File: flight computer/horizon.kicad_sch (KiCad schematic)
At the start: 36 parts, among them J2 Conn_02x03_Counter_Clockwise, J7 Conn_02x03_Counter_Clockwise, J8 Conn_02x03_Counter_Clockwise, U1 MMCU, U3 NMCU, U4 TMCU, Y1 Crystal

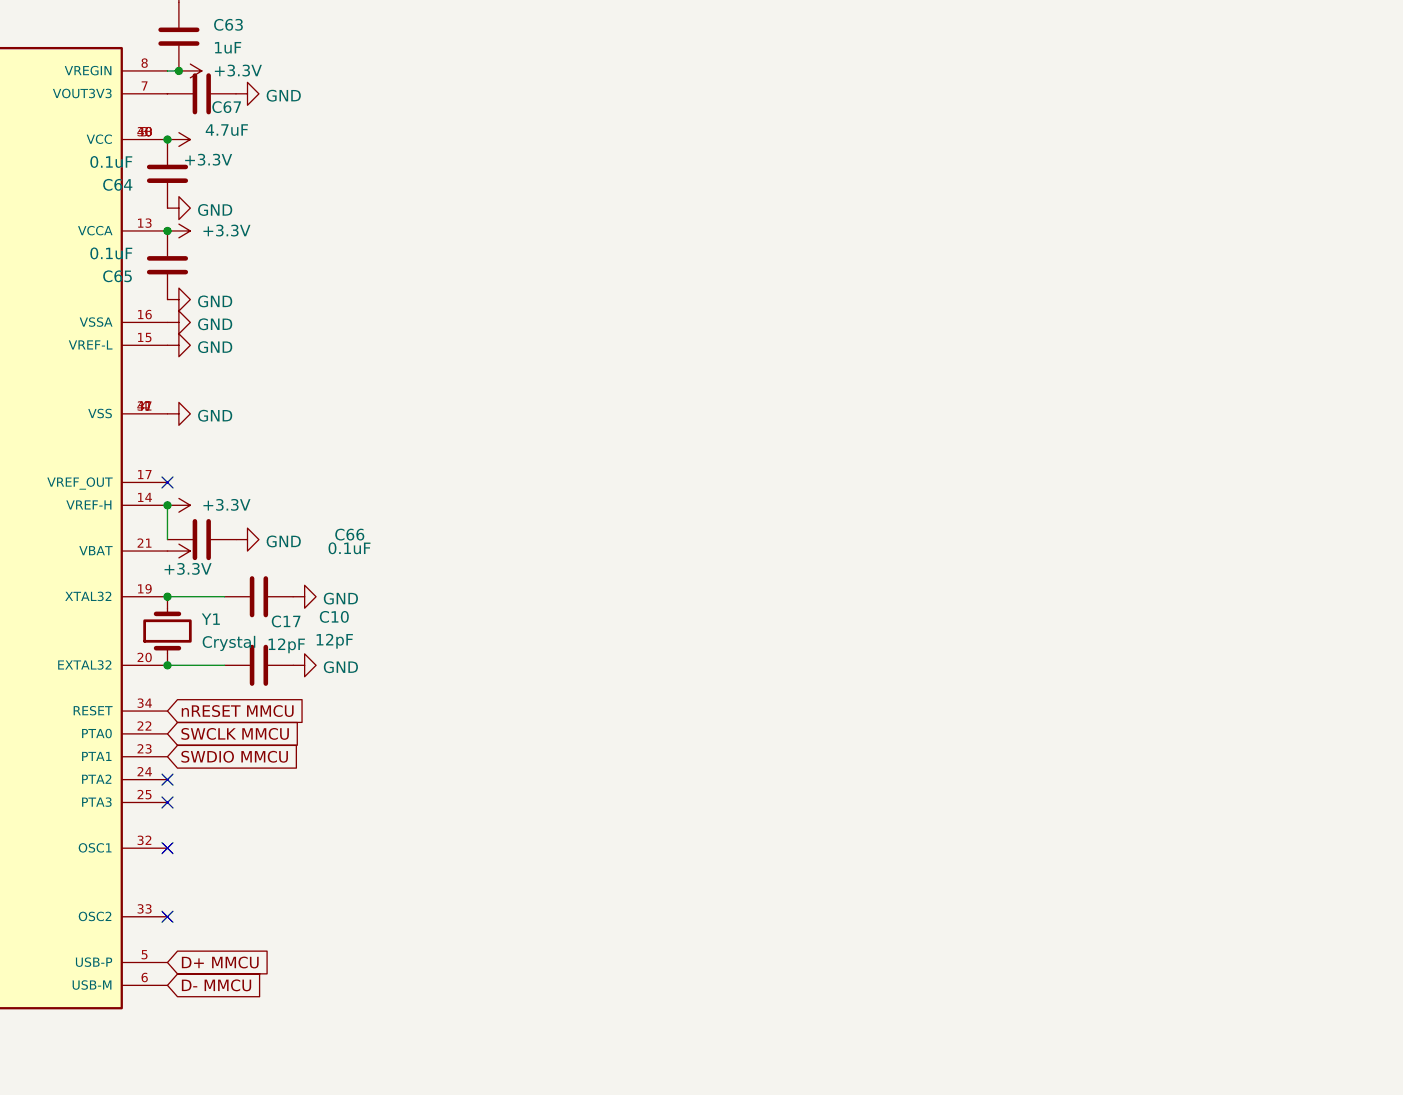
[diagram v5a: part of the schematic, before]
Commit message: Started wiring the teensy bootloader
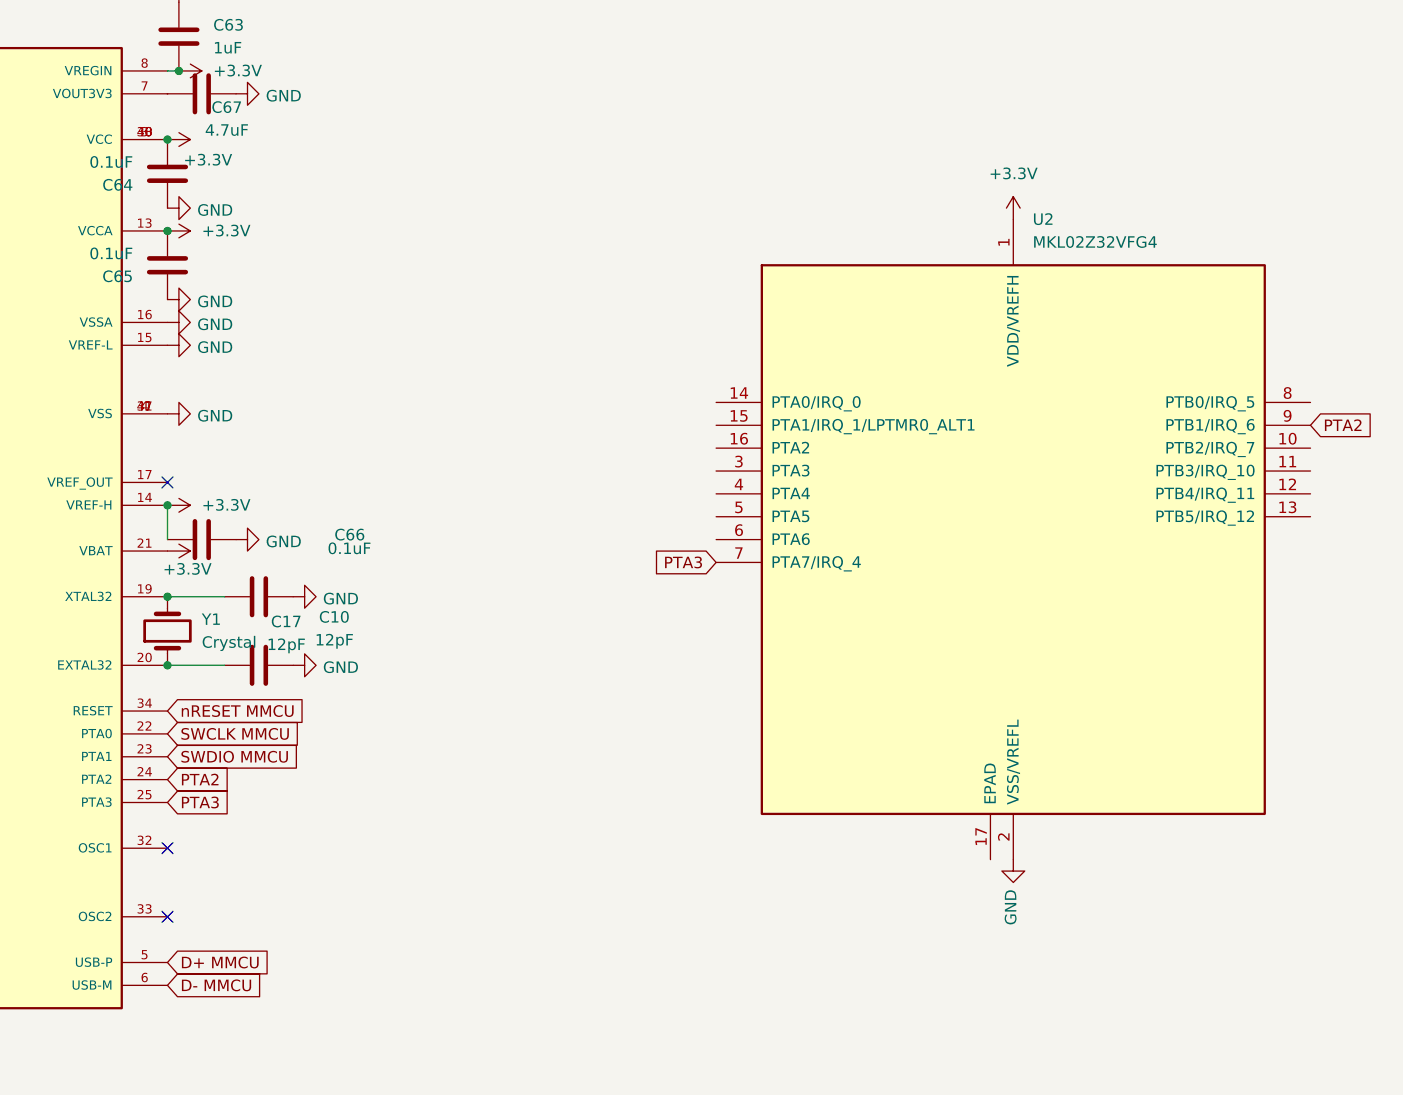
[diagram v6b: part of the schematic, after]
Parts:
- added U2: MKL02Z32VFG4, Package_DFN_QFN:QFN-16-1EP_3x3mm_P0.5mm_EP1.9x1.9mm, symbol MCU_NXP_Kinetis:MKL02Z32VFG4
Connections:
- net +3.3V: now also U2.1 (VDD/VREFH)
- net GND: now also U2.2 (VSS/VREFL)
- net PTA2: now reaches U1.24 (PTA2)
- net PTA2: now also U2.9 (PTB1/IRQ_6)
- net PTA3: now reaches U1.25 (PTA3)
- net PTA3: now also U2.7 (PTA7/IRQ_4)
- no-connect marks 79 -> 77
